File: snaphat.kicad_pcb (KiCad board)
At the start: 2 copper layers, 100 x 65.1 mm, 111 parts, among them J1 Conn_01x08_S8B-PH-K-S(LF)(SN), J2 Conn_02x20_2214SM-40G-75-PCR, J3 Conn_01x02_B2B-PH-K-S(LF)(SN), J4 USB_C_USB4125-GF-A-0190, J5 Conn_01x03_MC34747, Q1 Q_BC817-25, Q2 Q_NTR4003NT1G, Q3 Q_NTR4003NT1G, SW1 SW_B3FS-1050, SW2 SW_B3FS-1050, SW3 SW_B3FS-1050, SW4 SW_B3FS-1050, SW5 SW_B3FS-1050, SW6 SW_B3FS-1050, SW7 SW_B3FS-1050, SW8 SW_B3F-3150, U1 INA219BIDR, U2 MPQ3414BGJ-5-AEC1-P, U3 MCP73871T-2CCI/ML, U4 1825232-1, U5 AP9101CAK6-ABTRG1, U6 LIS2DW12TR

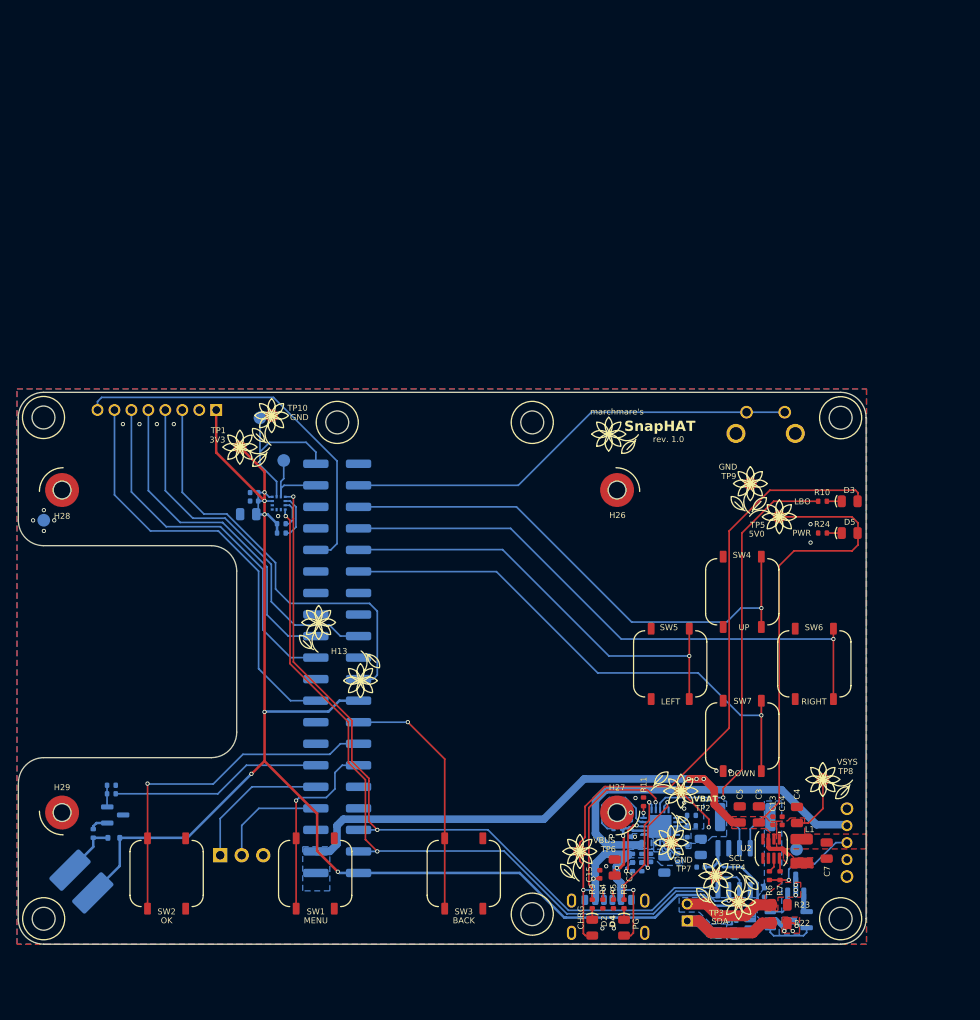
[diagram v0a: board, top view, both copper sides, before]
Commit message: Start updating PCB, library fixes
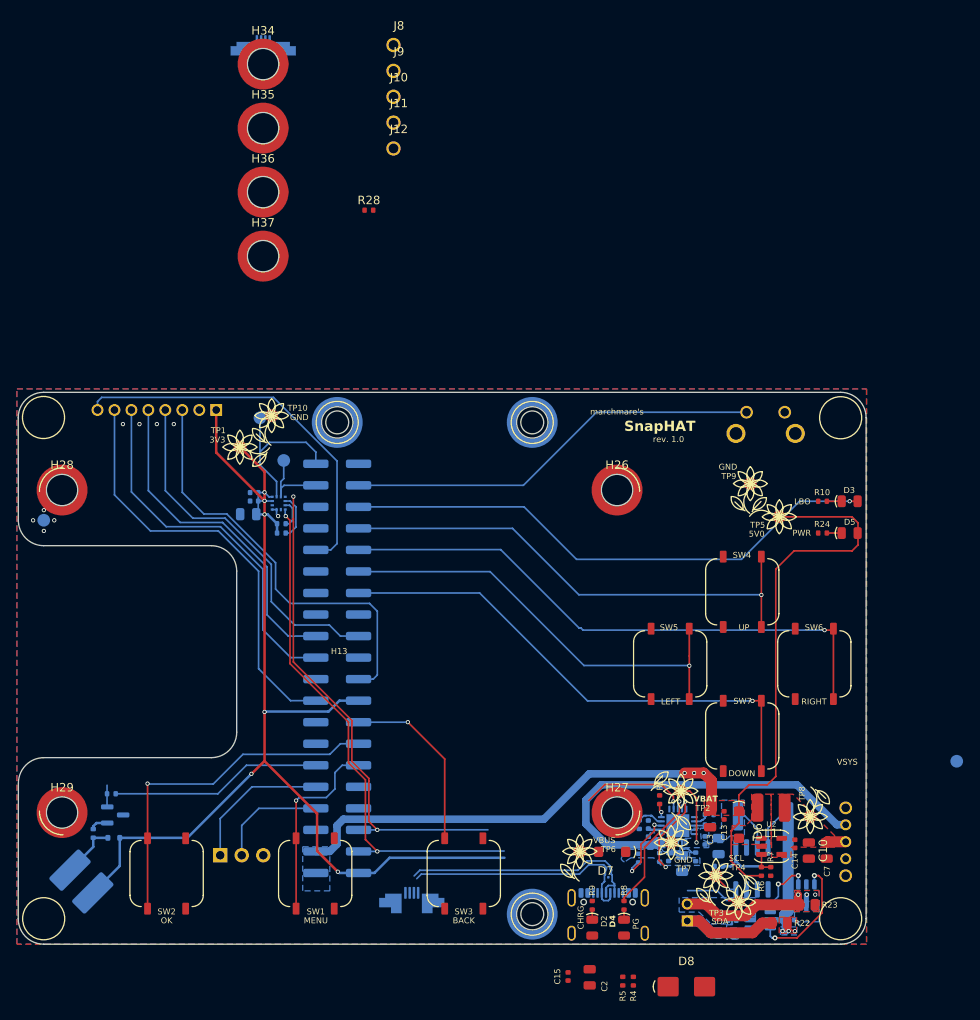
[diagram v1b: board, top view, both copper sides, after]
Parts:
- removed C4: 10u, library:C_0805_2012Metric
- removed C5: 1u, library:C_0805_2012Metric
- removed Q3: Q_NTR4003NT1G, library:SOT-23
- removed R17, R19: 0R, library:R_0402_1005Metric
- removed R2: 10k, library:R_0402_1005Metric
- removed REF** (x8): , library:TestPoint_Ornament
- removed REF** (x4): MountingHole_2.7mm, library:MountingHole_2.7mm
- added C10: 10u, library:C_0805_2012Metric, F.Cu at (239.9, 114.5)
- added D6: SL04-E3-08, library:DO-219AB, F.Cu at (231.7, 111.4)
- added D7: SL04-E3-08, library:DO-219AB, F.Cu at (216.7, 114.6)
- added D8: D_SMBJ5.0A, library:D_SMB, F.Cu at (225.4, 130.5)
- added H34: 9774020951R, library:Mounting_Wuerth_WA-SMST-2.7mm_H2mm_9774020951, F.Cu at (175.5, 21.7)
- added H35: 9774020951R, library:Mounting_Wuerth_WA-SMST-2.7mm_H2mm_9774020951, F.Cu at (175.5, 29.2)
- added H36: 9774020951R, library:Mounting_Wuerth_WA-SMST-2.7mm_H2mm_9774020951, F.Cu at (175.5, 36.8)
- added H37: 9774020951R, library:Mounting_Wuerth_WA-SMST-2.7mm_H2mm_9774020951, F.Cu at (175.5, 44.3)
- added J10: P70-6000045R, library:HARWIN_P70-6000045R, F.Cu at (190.9, 25.5)
- added J11: P70-6000045R, library:HARWIN_P70-6000045R, F.Cu at (190.9, 28.6)
- added J12: P70-6000045R, library:HARWIN_P70-6000045R, F.Cu at (190.9, 31.6)
- added J6: Conn_01x04_SFV4R-3STBE1HLF/C, library:AMPHENOL_SFV4R-3STBE1HLF, B.Cu at (193.1, 121.8)
- added J7: Conn_01x04_SFV4R-3STBE1HLF/C, library:AMPHENOL_SFV4R-3STBE1HLF, B.Cu at (175.5, 21.4)
- added J8: P70-6000045R, library:HARWIN_P70-6000045R, F.Cu at (190.9, 19.4)
- added J9: P70-6000045R, library:HARWIN_P70-6000045R, F.Cu at (190.9, 22.5)
- added R28: 330R, library:R_0402_1005Metric, F.Cu at (188.0, 38.9)
- added SW9: 1825232-1, library:1825232-1, B.Cu at (244.2, 113.4)
- C3: value 22u -> 2u2
- D2: value 0805 G LED -> 0805 B LED
- D4: value 0805 B LED -> 0805 R LED
- H15: value 803040 -> 10304
- H26, H27, H28, H29: value 9774030633R -> 9774030151R; footprint library:Mounting_Wuerth_WA-SMSI-M1.6_H3mm_9774030633 -> library:Mounting_Wuerth_WA-SMSI-M2.5_H3mm_9774030151R
- H30, H31, H32: value 970110151 -> 9774100151R; footprint library:970110151 -> library:Mounting_Wuerth_WA-SMSI-M2.5_H10mm_9774100151R
- J4: value USB_C_USB4125-GF-A-0190 -> USB_C_USB4930-00-A; footprint library:USB_C_Receptacle_GCT_USB4125-xx-x-0190_6P_TopMnt_Horizontal -> library:USB_C_Receptacle_GCT_USB4105-xx-A_16P_TopMnt_Horizontal
- L1: value L_SRP3212A-R68M -> L_LQH44PH100MPRL; footprint library:L_1210_3225Metric -> library:L_LPH44PH
- Q2: value Q_NTR4003NT1G -> Q_FDC6561AN; footprint library:SOT-23 -> library:SSOT-6
- R10: value 150R -> 47R
- R14: value 10k -> 2k7
- R6: value 10k -> 100k
- R7: value 10k -> 33k
- R9: value 150R -> 100R
- U2: value MPQ3414BGJ-5-AEC1-P -> MIC2250-1YD5-TR; footprint library:TSOT-23-8 -> library:TSOT-23-5
- U4: value 1825232-1 -> TPD2EUSB30DRTR; footprint library:1825232-1 -> library:Texas_DRT-3
- moved U4 28.4 mm to (216.2, 117.2), turned to 0 degrees
- moved TP11 21.6 mm to (257.3, 103.9)
- moved C2 13.3 mm to (214.1, 129.4)
- moved C15 12.6 mm to (211.5, 129.3)
- moved R4 9.79 mm to (219.2, 129.8), turned to 90 degrees
- moved R5 9.17 mm to (217.9, 129.8), turned to 90 degrees
- moved L1 6.25 mm to (235.4, 109.4), turned to 180 degrees
- moved C13 5.80 mm to (229.9, 110.3), turned to 90 degrees
- moved C3 5.78 mm to (228.2, 110.8), turned to -90 degrees
- moved TP8 4.62 mm to (240.1, 110.4), turned to 180 degrees
- moved R20 4.38 mm to (237.7, 122.6), turned to 180 degrees
- moved R23 3.25 mm to (239.7, 120.8)
- moved C14 3.10 mm to (238.2, 113.7), turned to 90 degrees
- moved R13 2.57 mm to (219.9, 111.4), turned to -90 degrees
- moved C21 2.11 mm to (221.0, 111.4)
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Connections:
- net +BATT renamed VBAT
- net ACCEL_INT1 renamed /ACCEL_INT1
- net ACCEL_INT2 renamed /ACCEL_INT2
- net BTN_BACK renamed /BTN_B
- net BTN_MENU renamed /BTN_MENU
- net BTN_OK renamed /BTN_A
- net CHARGING_STAT renamed /Power supply/CHRG_DONE_STAT
- net I2C_SCL renamed /I2C_SCL
- net I2C_SDA renamed /I2C_SDA
- net Net-(J3-Pin_1) renamed /Power supply/BATTERY_P
- net PROG1 renamed /Power supply/PROG1
- net PROG2 renamed /Power supply/PROG2
- net TIMER_EN renamed Net-(U3-~{TE})
- C15 pad 2: VBUS -> /USBC_VBUS_IN
- C17 pad 2: Net-(C17-Pad2) -> /Power supply/VOUT
- C2 pad 1: VBUS -> /USBC_VBUS_IN
- D3 pad 2: VBUS -> /LOW_BATTERY
- J1 pad 2: GND -> +5V
- J1 pad 5: DISPLAY_SPI_CS -> +5V
- J1 pad 6: DISPLAY_DC -> +5V
- J1 pad 7: DISPLAY_RST -> +5V
- J1 pad 8: DISPLAY_BL -> +5V
- J2 pad 10: RPI_UART_RX -> GND
- J2 pad 12: BUZZER_SIGNAL -> GND
- J2 pad 18: DISPLAY_RST -> GND
- J2 pad 19: DISPLAY_SPI_MOSI -> /DISPLAY_MOSI
- J2 pad 22: DISPLAY_DC -> GND
- J2 pad 23: DISPLAY_SPI_SCLK -> /DISPLAY_SPI_SCLK
- J2 pad 24: DISPLAY_SPI_CS -> GND
- J2 pad 27: unconnected-(J2-Pin_27-Pad27) -> /BTN_D
- J2 pad 29: BTN_D -> /BTN_L
- J2 pad 31: BTN_L -> /BTN_R
- J2 pad 32: DISPLAY_BL -> GND
- J2 pad 33: BTN_R -> /BTN_U
- J2 pad 35: BTN_U -> /LOW_BATTERY
- J2 pad 37: BTN_SHUTTER -> /BTN_SHUTTER
- J2 pad 8: RPI_UART_TX -> GND
- J4 pad A9: VBUS -> /USBC_VBUS_IN
- J4 pad B9: VBUS -> /USBC_VBUS_IN
- J5 pad 1: RPI_UART_RX -> GND
- J5 pad 2: RPI_UART_TX -> GND
- L1 pad 2: Net-(U2-SW) -> Net-(D6-A)
- Q1 pad 1: Net-(Q1-C) -> Net-(Q1-B)
- Q1 pad 2: Net-(Q1-B) -> GND
- Q1 pad 3: GND -> Net-(BZ1--)
- Q2 pad 1: Net-(Q2-D) -> Net-(U5-DO)
- Q2 pad 2: Net-(Q2-G) -> GND
- Q2 pad 3: GNDS -> Net-(U5-CO)
- R1 pad 1: BUZZER_SIGNAL -> GND
- R10 pad 1: LBO_STAT -> GND
- R14 pad 1: PROG3 -> GND
- R14 pad 2: GND -> /Power supply/PROG3
- R18 pad 1: PS_SELECT -> VBUS
- R18 pad 2: VBUS -> Net-(U3-SEL)
- R27 pad 1: Net-(BZ1--) -> /GND_EXT
- R27 pad 2: Net-(Q1-C) -> /OTG_EXT
- R4 pad 1: Net-(J4-CC2) -> GND
- R4 pad 2: GND -> Net-(J4-CC1)
- R5 pad 1: Net-(J4-CC1) -> GND
- R5 pad 2: GND -> Net-(J4-CC2)
- R6 pad 1: VSYS -> +5V
- R6 pad 2: Net-(U2-MODE) -> Net-(U2-FB)
- R7 pad 1: VSYS -> Net-(U2-FB)
- R7 pad 2: Net-(U2-EN) -> GND
- R8 pad 1: POWER_GOOD -> /Power supply/CHRG_STAT
- SW4 pad 1: BTN_U -> /BTN_U
- SW4 pad 2: BTN_U -> /BTN_U
- SW5 pad 1: BTN_L -> /BTN_L
- SW5 pad 2: BTN_L -> /BTN_L
- SW6 pad 1: BTN_R -> /BTN_R
- SW6 pad 2: BTN_R -> /BTN_R
- SW7 pad 1: BTN_D -> /BTN_D
- SW7 pad 2: BTN_D -> /BTN_D
- SW8 pad 1: BTN_SHUTTER -> /BTN_SHUTTER
- SW8 pad 2: BTN_SHUTTER -> GND
- U2 pad 1: VSYS -> Net-(D6-A)
- U2 pad 2: +5V -> GND
- U2 pad 3: Net-(U2-SW) -> Net-(U2-FB)
- U2 pad 4: GND -> VSYS
- U2 pad 5: GND -> VSYS
- U3 pad 1: Net-(C17-Pad2) -> /Power supply/VOUT
- U3 pad 12: PROG3 -> /Power supply/PROG3
- U3 pad 20: Net-(C17-Pad2) -> /Power supply/VOUT
- U3 pad 3: PS_SELECT -> Net-(U3-SEL)
- U3 pad 6: POWER_GOOD -> unconnected-(U3-~{PG}-Pad6)
- U3 pad 8: LBO_STAT -> /Power supply/CHRG_STAT
- U4 pad 1: Net-(C17-Pad2) -> /USBC_DATA_P
- U4 pad 2: VSYS -> /USBC_DATA_N
- U4 pad 3: unconnected-(U4-Pad3) -> GND
- U5 pad 1: Net-(Q2-G) -> Net-(U5-DO)
- U5 pad 3: Net-(Q3-G) -> Net-(U5-CO)
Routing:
- net +5V: track 113.5 -> 304.9 mm, vias 3 -> 11
- net VBUS: track 112.9 -> 3.99 mm, vias 5 -> 0
- net BTN_R: track 69.7 -> 0.00 mm, vias 1 -> 0
- net /BTN_R: track 0.00 -> 68.3 mm, vias 0 -> 1
- net /LOW_BATTERY: track 0.00 -> 64.3 mm, vias 0 -> 1
- net BTN_D: track 62.8 -> 0.00 mm, vias 1 -> 0
- net BTN_U: track 62.1 -> 0.00 mm, vias 1 -> 0
- net /BTN_D: track 0.00 -> 61.1 mm, vias 0 -> 1
- net /BTN_U: track 0.00 -> 59.1 mm, vias 0 -> 1
- net GND: track 42.0 -> 97.6 mm, vias 22 -> 1
- net BTN_SHUTTER: track 53.8 -> 0.00 mm
- net BTN_L: track 52.5 -> 0.00 mm, vias 1 -> 0
- net /BTN_L: track 0.00 -> 51.9 mm, vias 0 -> 1
- net LBO_STAT: track 51.2 -> 0.00 mm, vias 1 -> 0
- net DISPLAY_RST: track 50.6 -> 0.00 mm
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- added copper zone on B.Cu, net /Power supply/VOUT
- added copper zone on F.Cu, net Net-(D6-A)
- added copper zone on B.Cu, net Net-(Q2-Pad4)
- removed copper zone on B.Cu, net Net-(C17-Pad2)
- removed copper zone on F.Cu, net Net-(U2-SW)
